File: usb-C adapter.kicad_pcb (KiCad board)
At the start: 2 copper layers, 88.3 x 78.1 mm, 65 parts, among them U1 IP2721, U2 LND01

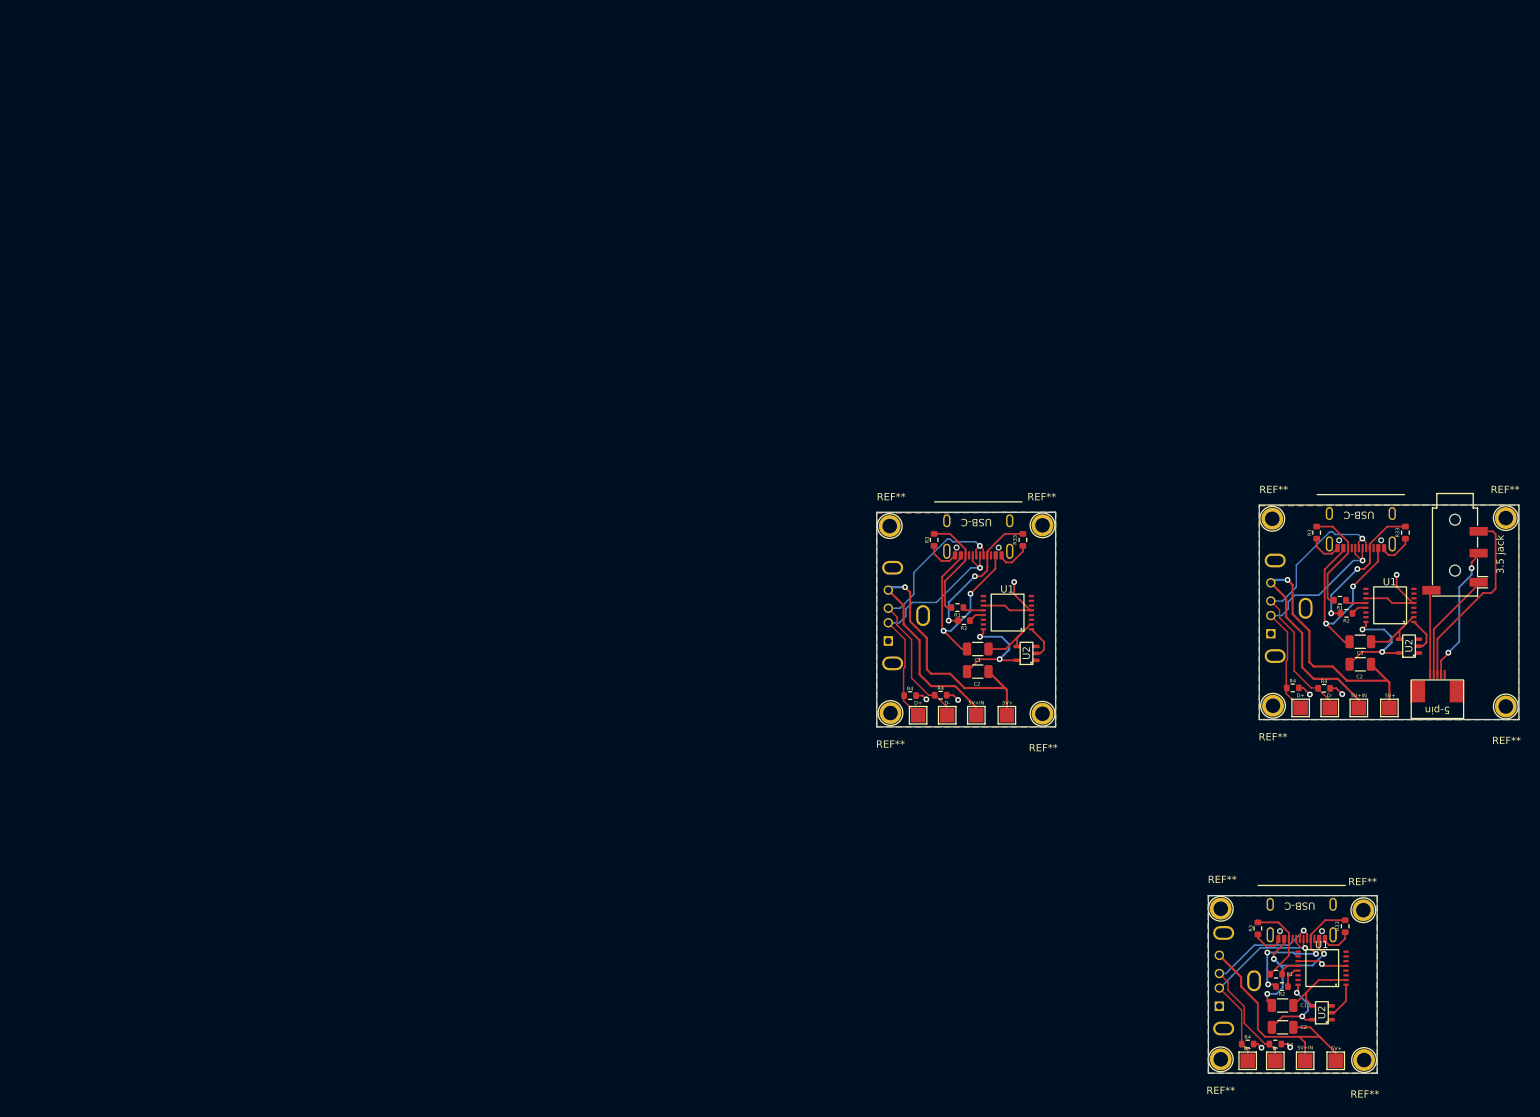
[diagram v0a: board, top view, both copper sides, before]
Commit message: build(2.0-build-with-reduced-size-and-cleaned-contact-points): no
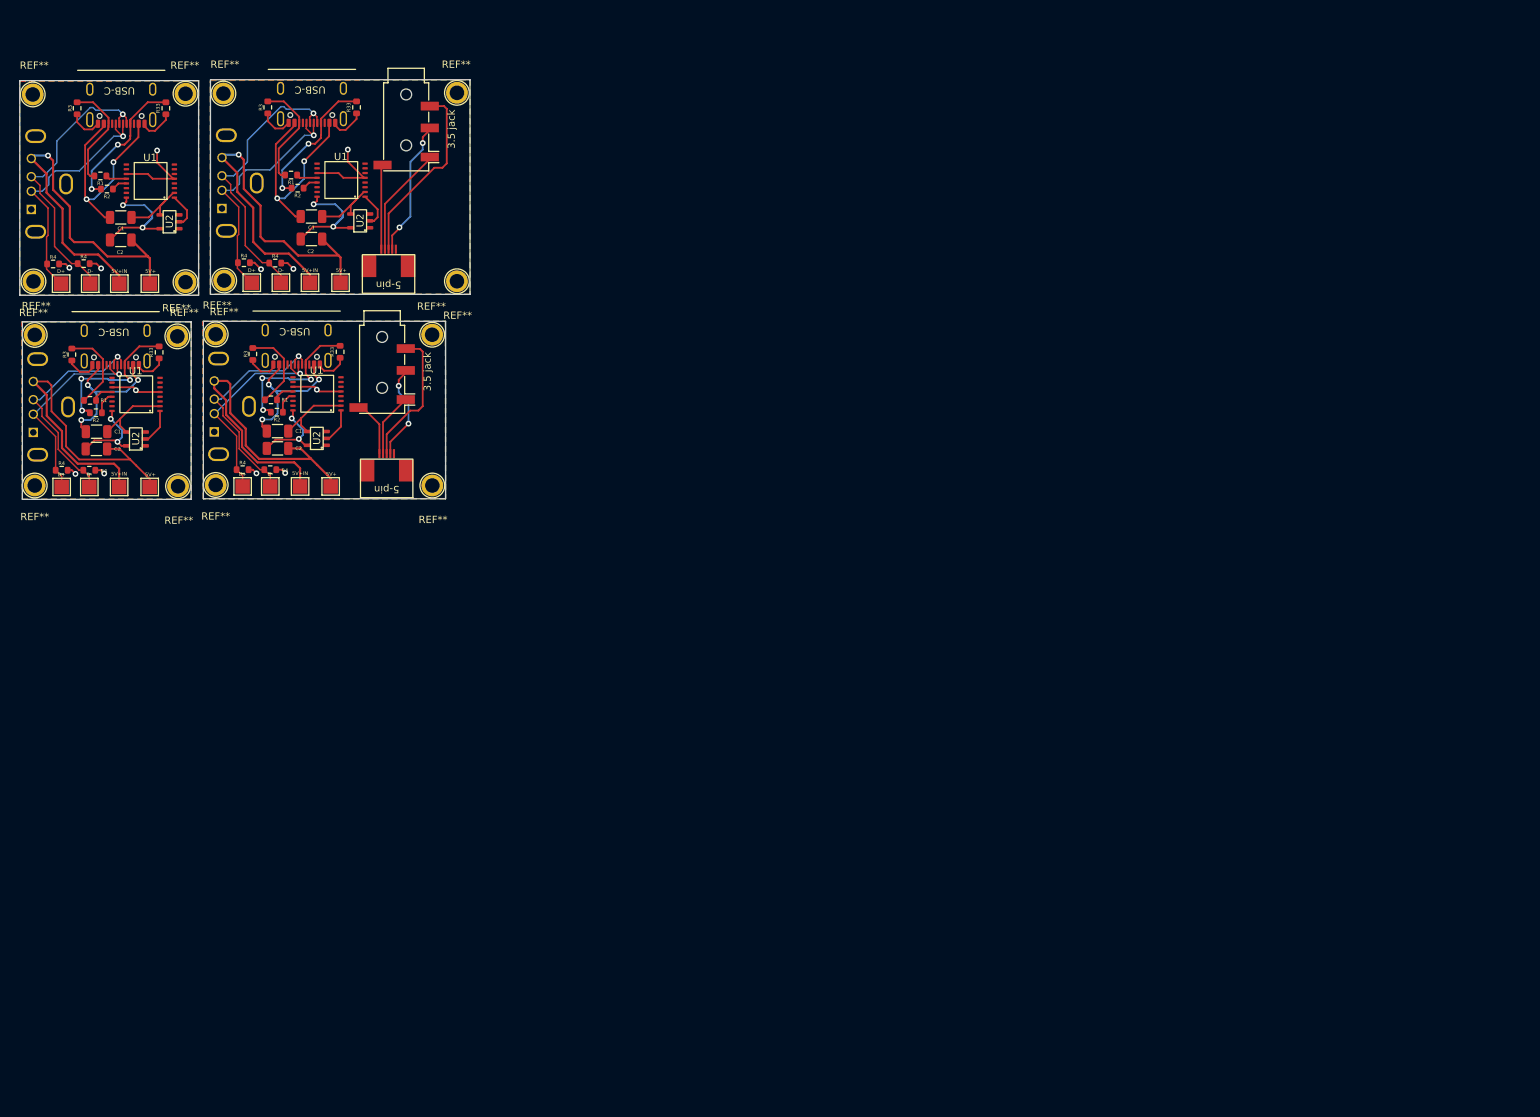
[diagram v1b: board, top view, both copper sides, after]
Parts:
- added 3.5 jack: Jack_3.5mm_PJ320D_Horizontal, Connector_Audio:Jack_3.5mm_PJ320D_Horizontal, F.Cu at (63.2, 52.8)
- added 5-pin: 5pin FPC, ucb-c adapter:5pin FPC, F.Cu at (63.9, 67.5)
- added 5V+: TestPoint_Pad_2.0x2.0mm, TestPoint:TestPoint_Pad_2.0x2.0mm, F.Cu at (56.1, 68.5)
- added 5V+IN: TestPoint_Pad_2.0x2.0mm, TestPoint:TestPoint_Pad_2.0x2.0mm, F.Cu at (52.0, 68.5)
- added C1: C_1206_3216Metric, Capacitor_SMD:C_1206_3216Metric, F.Cu at (48.9, 61.0)
- added C2: C_1206_3216Metric, Capacitor_SMD:C_1206_3216Metric, F.Cu at (48.9, 63.3)
- added D+: TestPoint_Pad_2.0x2.0mm, TestPoint:TestPoint_Pad_2.0x2.0mm, F.Cu at (44.0, 68.5)
- added D-: TestPoint_Pad_2.0x2.0mm, TestPoint:TestPoint_Pad_2.0x2.0mm, F.Cu at (47.9, 68.5)
- added G***: LOGO, graphics:iblis 5mm, B.Cu at (59.1, 62.0)
- added R1: R_0603_1608Metric, Resistor_SMD:R_0603_1608Metric, F.Cu at (48.0, 56.6)
- added R2: R_0603_1608Metric, Resistor_SMD:R_0603_1608Metric, F.Cu at (48.8, 58.4)
- added R3: R_0603_1608Metric, Resistor_SMD:R_0603_1608Metric, F.Cu at (45.5, 50.4)
- added R33: R_0603_1608Metric, Resistor_SMD:R_0603_1608Metric, F.Cu at (57.5, 50.0)
- added R4: R_0603_1608Metric, Resistor_SMD:R_0603_1608Metric, F.Cu at (44.0, 66.2)
- added R4: R_0603_1608Metric, Resistor_SMD:R_0603_1608Metric, F.Cu at (47.9, 66.2)
- added REF**: TestPoint_Plated_Hole_D2.0mm, TestPoint:TestPoint_Plated_Hole_D2.0mm, F.Cu at (70.1, 47.7)
- added REF**: TestPoint_Plated_Hole_D2.0mm, TestPoint:TestPoint_Plated_Hole_D2.0mm, F.Cu at (70.1, 68.4)
- added REF**: TestPoint_Plated_Hole_D2.0mm, TestPoint:TestPoint_Plated_Hole_D2.0mm, F.Cu at (40.4, 47.6)
- added REF**: TestPoint_Plated_Hole_D2.0mm, TestPoint:TestPoint_Plated_Hole_D2.0mm, F.Cu at (40.4, 68.3)
- added U1: IP2721, ucb-c adapter:IP2721, F.Cu at (54.3, 55.8)
- added U2: LND01, ucb-c adapter:LND01, F.Cu at (54.2, 62.0)
- added USB-A: USB_A_Molex_105057_Vertical, Connector_USB:USB_A_Molex_105057_Vertical, B.Cu at (40.1, 61.0)
- added USB-C: usb-c f, ucb-c adapter:usb-c f, F.Cu at (51.5, 48.4)
- moved C2 181.4 mm to (23.9, 63.4)
- moved 5V+ 181.1 mm to (31.3, 68.6)
- moved 5V+IN 181.1 mm to (27.1, 68.6)
- moved C1 181.1 mm to (24.0, 61.0)
- moved D- 181.1 mm to (23.0, 68.6)
- moved G*** 181.1 mm to (32.5, 57.3)
- moved R1 181.1 mm to (23.1, 56.7)
- moved R2 181.1 mm to (23.9, 58.4)
- moved R3 181.1 mm to (20.6, 50.4)
- moved R4 181.1 mm to (23.0, 66.3)
- moved REF** 181.1 mm to (15.5, 68.4)
- moved REF** 181.1 mm to (15.5, 47.7)
- moved U2 181.1 mm to (29.4, 62.0)
- moved USB-A 181.1 mm to (15.3, 61.1)
- moved USB-C 181.1 mm to (26.6, 48.5)
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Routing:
- net 5V+: track 150.4 -> 222.0 mm
- net VBUS: track 124.3 -> 157.9 mm, vias 13 -> 18
- net D-: track 115.2 -> 147.8 mm, vias 3 -> 4
- net D+: track 97.8 -> 126.9 mm, vias 3 -> 4
- net GND: track 80.6 -> 107.1 mm, vias 9 -> 12
- net CC1: track 69.0 -> 93.2 mm, vias 7 -> 10
- net HRP: track 25.5 -> 44.4 mm
- net CC2: track 50.5 -> 65.6 mm
- net HPL: track 18.9 -> 32.4 mm, vias 2 -> 4
- net VIN: track 29.5 -> 40.3 mm
- net HPS: track 15.3 -> 24.1 mm
- net VBUSG: track 14.6 -> 19.5 mm
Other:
- board size 88.3 x 78.1 mm -> 61.9 x 57.7 mm

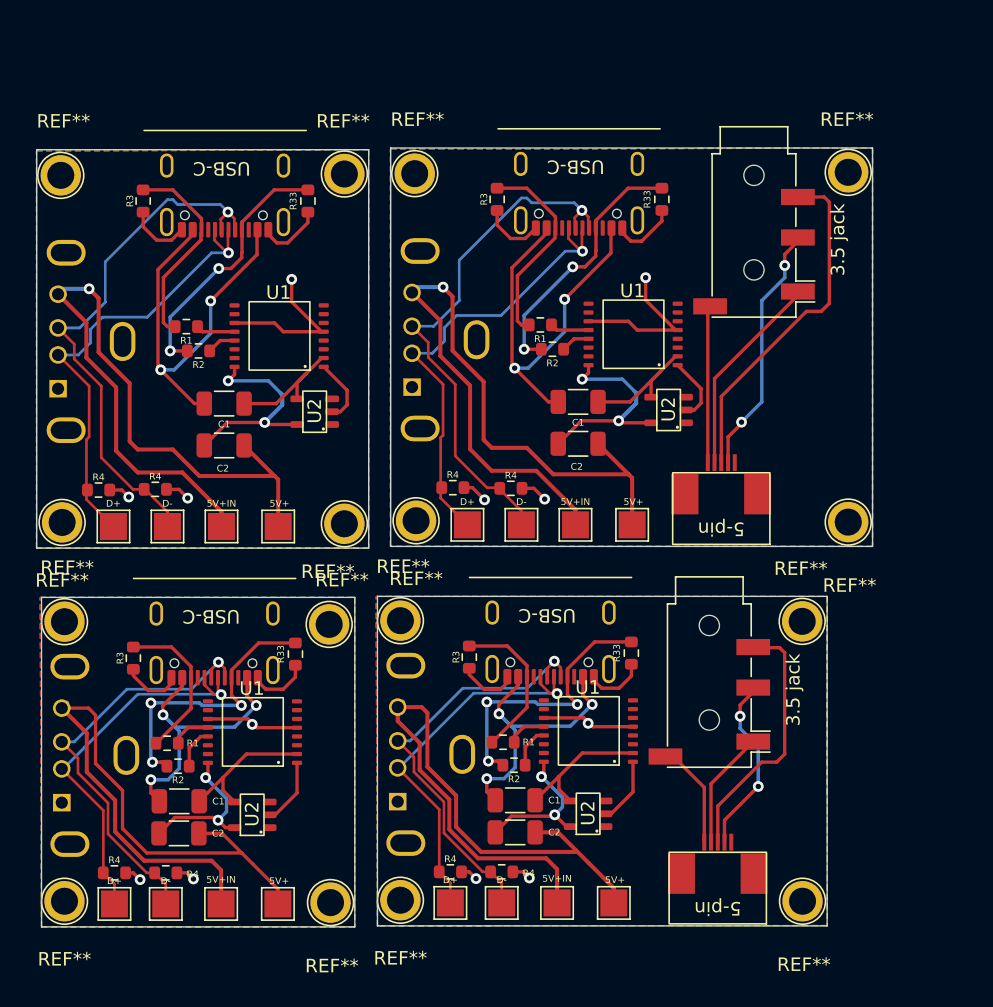
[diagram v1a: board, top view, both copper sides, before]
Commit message: build(final-push): final push
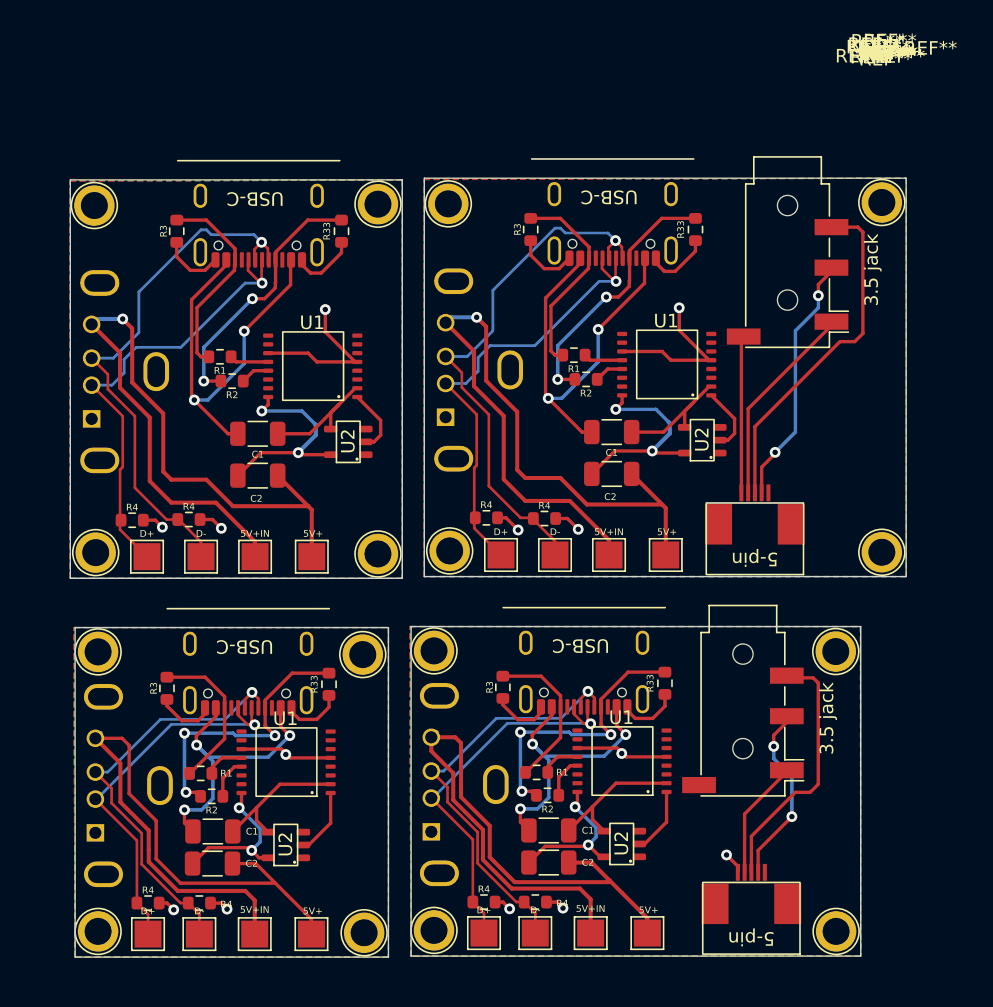
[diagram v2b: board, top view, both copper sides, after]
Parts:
- moved C2 3.34 mm to (26.4, 65.6)
- moved D+ 3.34 mm to (46.5, 70.8)
- moved R2 3.34 mm to (54.1, 29.8)
- moved R4 3.34 mm to (46.5, 68.5)
- moved REF** 3.34 mm to (37.7, 70.8)
- moved U1 3.34 mm to (60.1, 28.7)
- moved U1 3.34 mm to (56.8, 58.1)
- moved U2 3.34 mm to (31.9, 64.3)
- moved USB-C 3.34 mm to (54.0, 50.6)
- moved 5V+ 3.34 mm to (33.8, 42.9)
- moved 5V+IN 3.34 mm to (29.6, 70.9)
- moved C1 3.34 mm to (29.8, 33.8)
- moved R1 3.34 mm to (25.6, 59.0)
- moved R1 3.34 mm to (53.2, 28.0)
- moved R2 3.34 mm to (26.4, 60.7)
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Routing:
- net GND: track 107.1 -> 101.4 mm, vias 12 -> 13
